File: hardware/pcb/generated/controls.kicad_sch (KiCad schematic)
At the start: 22 parts, among them J1 PPPC202LFBN-RC, J2 PPPC041LFBN-RC, SW1 TL1105SPF100QG, SW10 TL1105SPF100QG, SW11 TL1105SPF100QG, SW12 TL1105SPF100QG, SW2 TL1105SPF100QG, SW3 TL1105SPF100QG, SW4 TL1105SPF100QG, SW5 TL1105SPF100QG, SW6 TL1105SPF100QG, SW7 TL1105SPF100QG, SW8 TL1105SPF100QG, SW9 TL1105SPF100QG, U5 SN74AHCT125DR

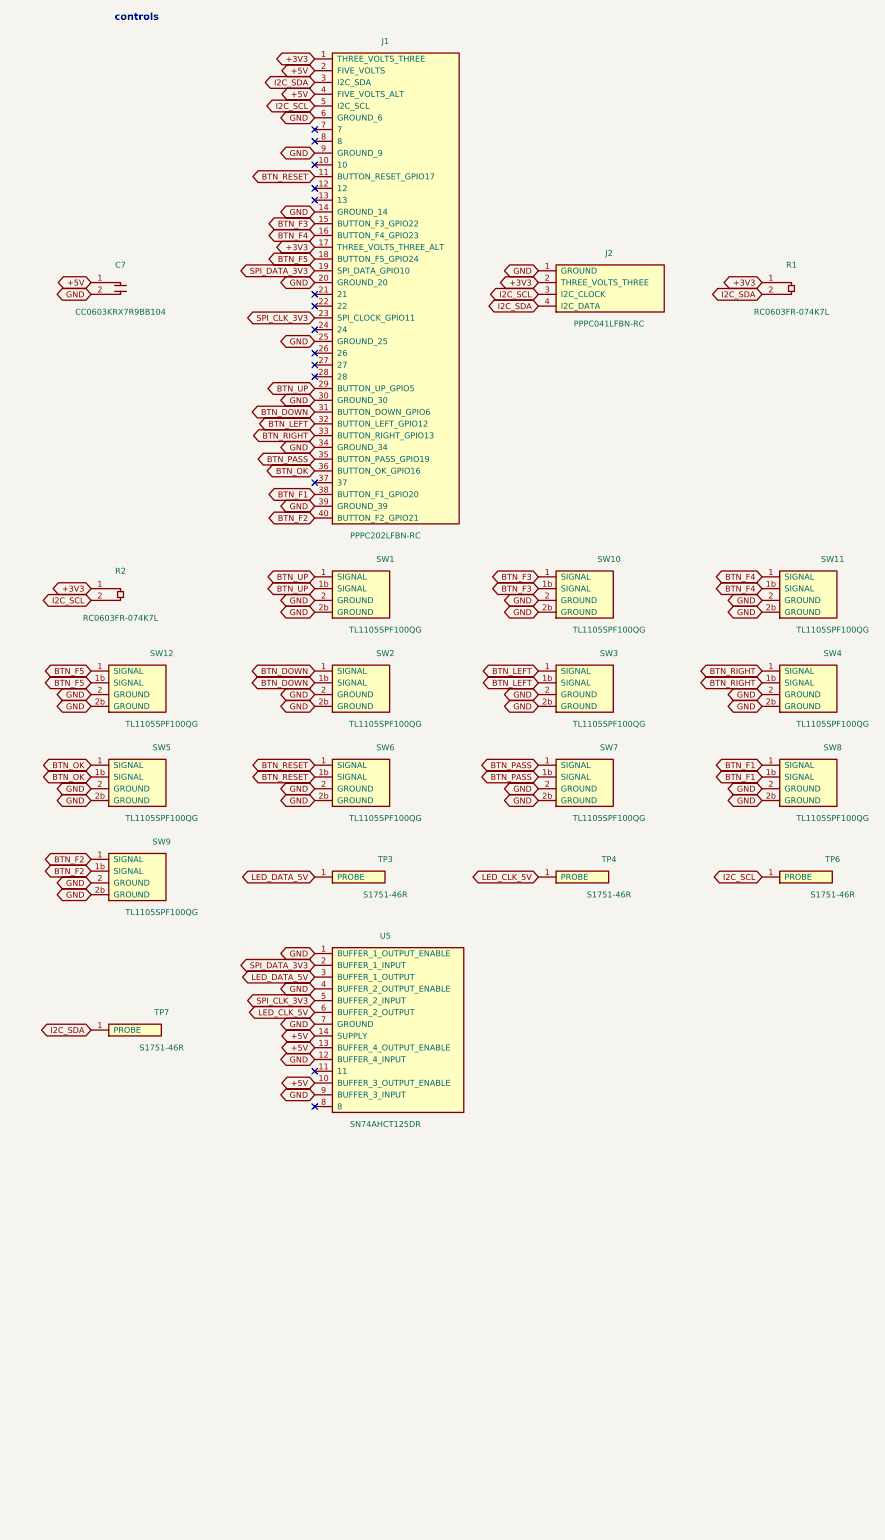
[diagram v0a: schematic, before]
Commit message: chore(pcb): regenerate KiCad, SPICE and review output
Generated by `just pcb` from the committed definition; not hand-edited.
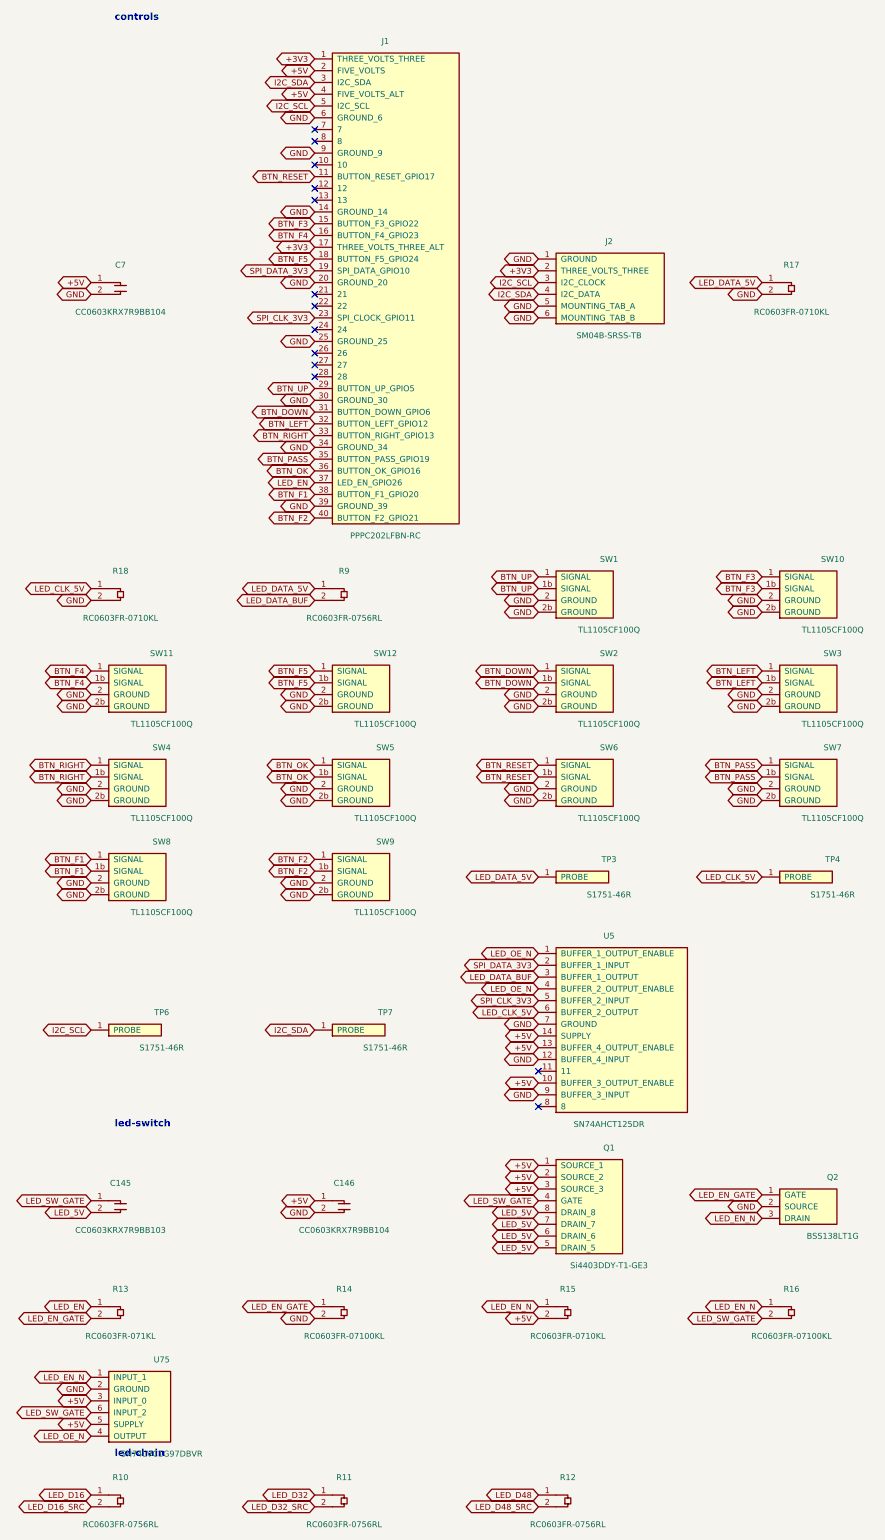
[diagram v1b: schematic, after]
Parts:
- removed R1: RC0603FR-074K7L, symbol Generated:R1
- removed R2: RC0603FR-074K7L, symbol Generated:R2
- added C145: CC0603KRX7R9BB103, symbol Generated:C145
- added C146: CC0603KRX7R9BB104, symbol Generated:C146
- added Q1: Si4403DDY-T1-GE3, symbol Generated:Q1
- added Q2: BSS138LT1G, symbol Generated:Q2
- added R10: RC0603FR-0756RL, symbol Generated:R10
- added R11: RC0603FR-0756RL, symbol Generated:R11
- added R12: RC0603FR-0756RL, symbol Generated:R12
- added R13: RC0603FR-071KL, symbol Generated:R13
- added R14: RC0603FR-07100KL, symbol Generated:R14
- added R15: RC0603FR-0710KL, symbol Generated:R15
- added R16: RC0603FR-07100KL, symbol Generated:R16
- added R17: RC0603FR-0710KL, symbol Generated:R17
- added R18: RC0603FR-0710KL, symbol Generated:R18
- added R9: RC0603FR-0756RL, symbol Generated:R9
- added U75: SN74LVC1G97DBVR, symbol Generated:U75
- J2: value PPPC041LFBN-RC -> SM04B-SRSS-TB
- SW1, SW10, SW11, SW12, SW2, SW3, SW4, SW5, SW6, SW7, SW8, SW9: value TL1105SPF100QG -> TL1105CF100Q
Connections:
- net +5V: now also C146.1 (SUPPLY_OR_ELECTRODE_A), Q1.1 (SOURCE_1), Q1.2 (SOURCE_2), Q1.3 (SOURCE_3), R15.2 (TERMINAL_B), U75.3 (INPUT_0), U75.5 (SUPPLY)
- net GND: now also J2.5 (MOUNTING_TAB_A), J2.6 (MOUNTING_TAB_B), C146.2 (RETURN_OR_ELECTRODE_B), Q2.2 (SOURCE), R14.2 (TERMINAL_B), R17.2 (TERMINAL_B), R18.2 (TERMINAL_B), U75.2 (GROUND); no longer U5.1 (BUFFER_1_OUTPUT_ENABLE), U5.4 (BUFFER_2_OUTPUT_ENABLE)
- net LED_CLK_5V: now also R18.1 (TERMINAL_A)
- net LED_DATA_5V: now also R17.1 (TERMINAL_A), R9.1 (TERMINAL_A); no longer U5.3 (BUFFER_1_OUTPUT)
- net LED_EN: now reaches J1.37 (LED_EN_GPIO26)
- net LED_EN: now also R13.1 (TERMINAL_A)
- new net LED_5V: C145.2 (RETURN_OR_ELECTRODE_B), Q1.5 (DRAIN_5), Q1.6 (DRAIN_6), Q1.7 (DRAIN_7), Q1.8 (DRAIN_8)
- new net LED_D16: R10.1 (TERMINAL_A)
- new net LED_D16_SRC: R10.2 (TERMINAL_B)
- new net LED_D32: R11.1 (TERMINAL_A)
- new net LED_D32_SRC: R11.2 (TERMINAL_B)
- new net LED_D48: R12.1 (TERMINAL_A)
- new net LED_D48_SRC: R12.2 (TERMINAL_B)
- new net LED_DATA_BUF: R9.2 (TERMINAL_B), U5.3 (BUFFER_1_OUTPUT)
- new net LED_EN_GATE: Q2.1 (GATE), R13.2 (TERMINAL_B), R14.1 (TERMINAL_A)
- new net LED_EN_N: Q2.3 (DRAIN), R15.1 (TERMINAL_A), R16.1 (TERMINAL_A), U75.1 (INPUT_1)
- new net LED_OE_N: U5.1 (BUFFER_1_OUTPUT_ENABLE), U5.4 (BUFFER_2_OUTPUT_ENABLE), U75.4 (OUTPUT)
- new net LED_SW_GATE: C145.1 (SUPPLY_OR_ELECTRODE_A), Q1.4 (GATE), R16.2 (TERMINAL_B), U75.6 (INPUT_2)
- no-connect marks 14 -> 13
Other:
- note added: "led-chain"
- note added: "led-switch"
- moved on the sheet: SW1, SW10, SW11, SW12, SW2, SW3, SW4, SW5, SW6, SW7, SW8, SW9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
